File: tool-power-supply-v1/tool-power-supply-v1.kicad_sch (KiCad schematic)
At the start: 0 parts

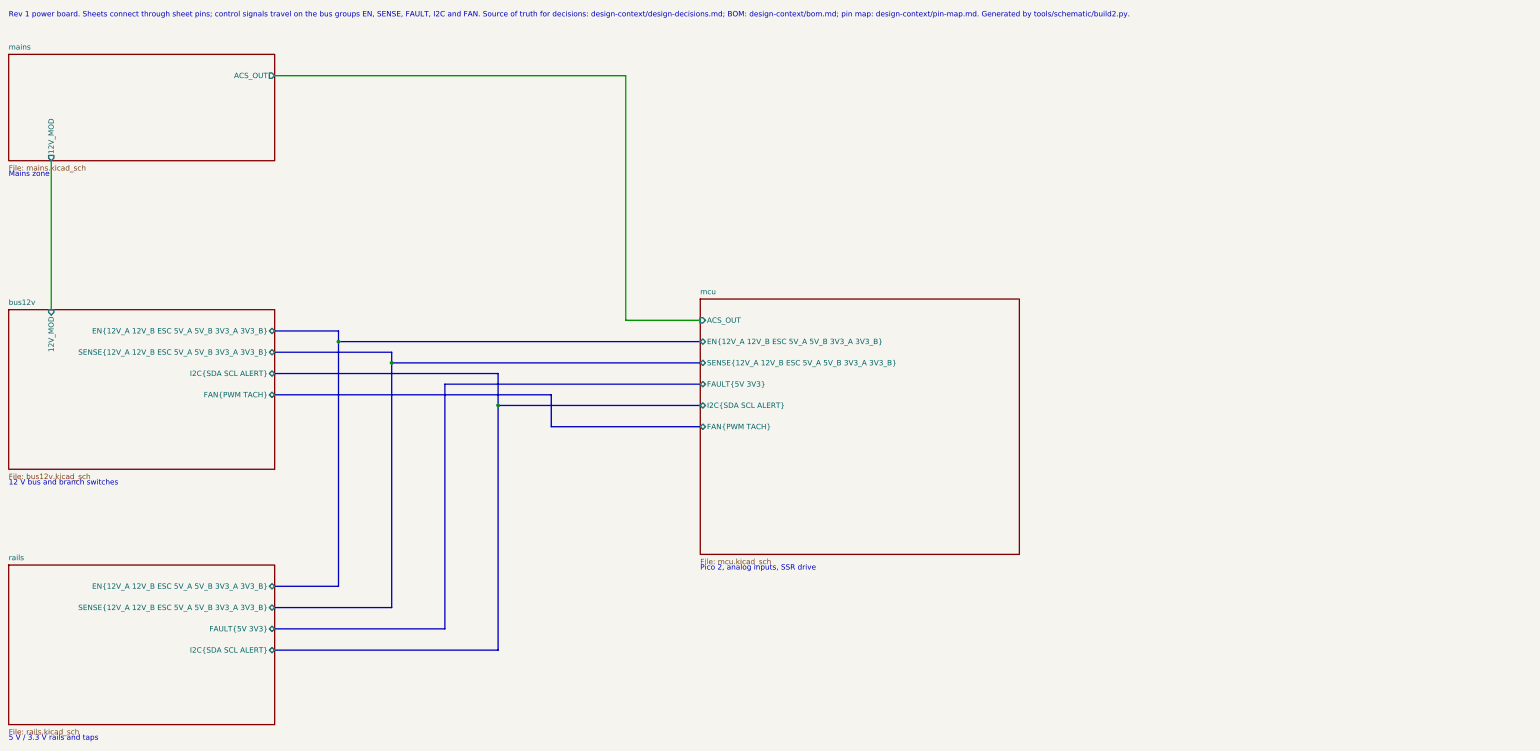
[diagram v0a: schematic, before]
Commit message: schematic update: finished cleaning up
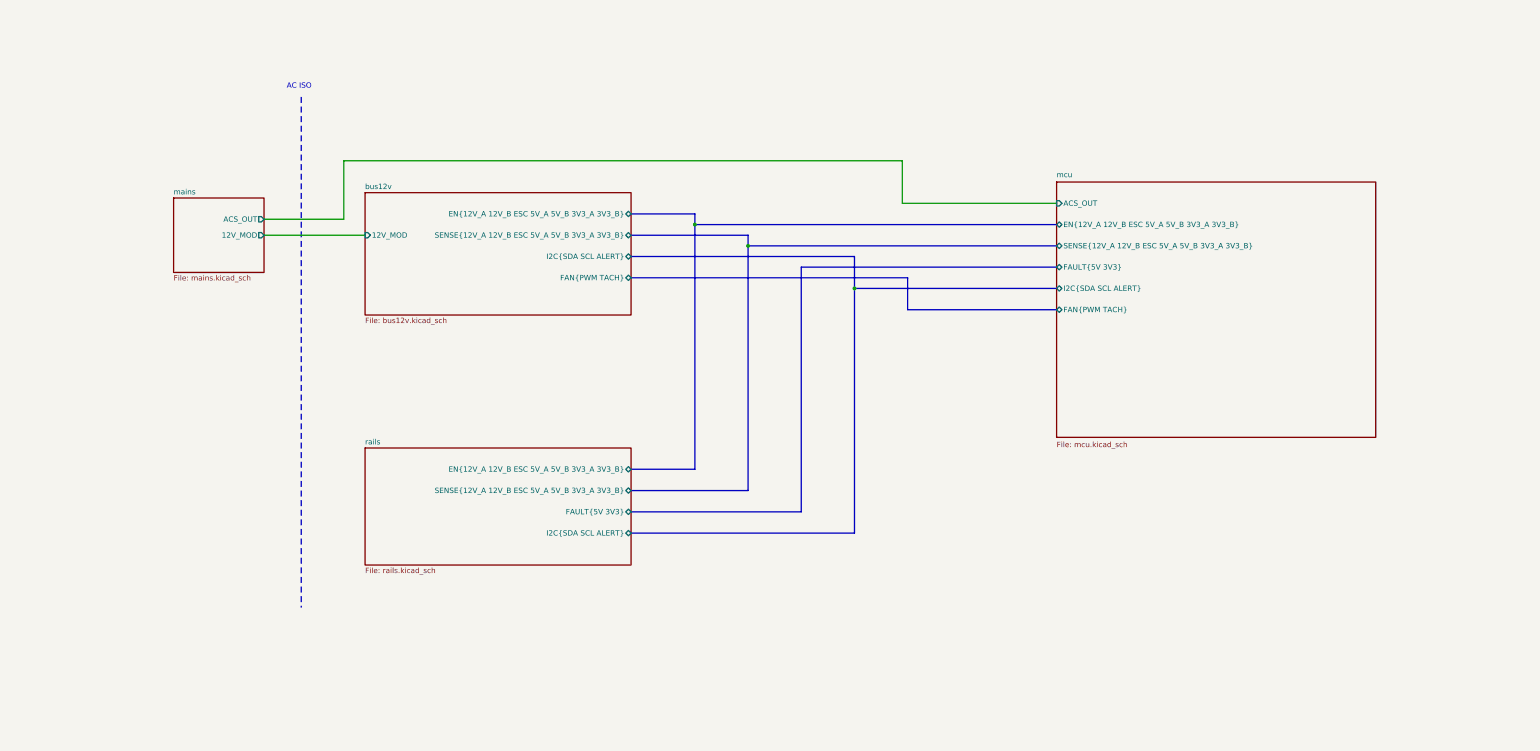
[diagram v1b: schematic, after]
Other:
- note added: "AC ISO"
- note removed: "12 V bus and branch switches"
- note removed: "5 V / 3.3 V rails and taps"
- note removed: "Mains zone"
- note removed: "Pico 2, analog inputs, SSR drive"
- note removed: "Rev 1 power board. Sheets connect through sheet pins; control signals travel on the bus groups EN, SENSE, FAULT, I2C and FAN. Source of truth for decisions: design-context/design-decisions.md; BOM: design-context/bom.md; pin map: design-context/pin-map.md. Generated by tools/schematic/build2.py."
